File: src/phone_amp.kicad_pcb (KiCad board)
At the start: 2 copper layers, 11.6 x 56.1 mm, 41 parts, among them J1 M_USB_B, J2 PJ313D, J3 PJ313D, J4 RJ9_4P4C, J5 RJ9_4P4C, SW1 SWITCH_INV, U1 TPA6139A2, U2 MCP6024, U3 TC1017

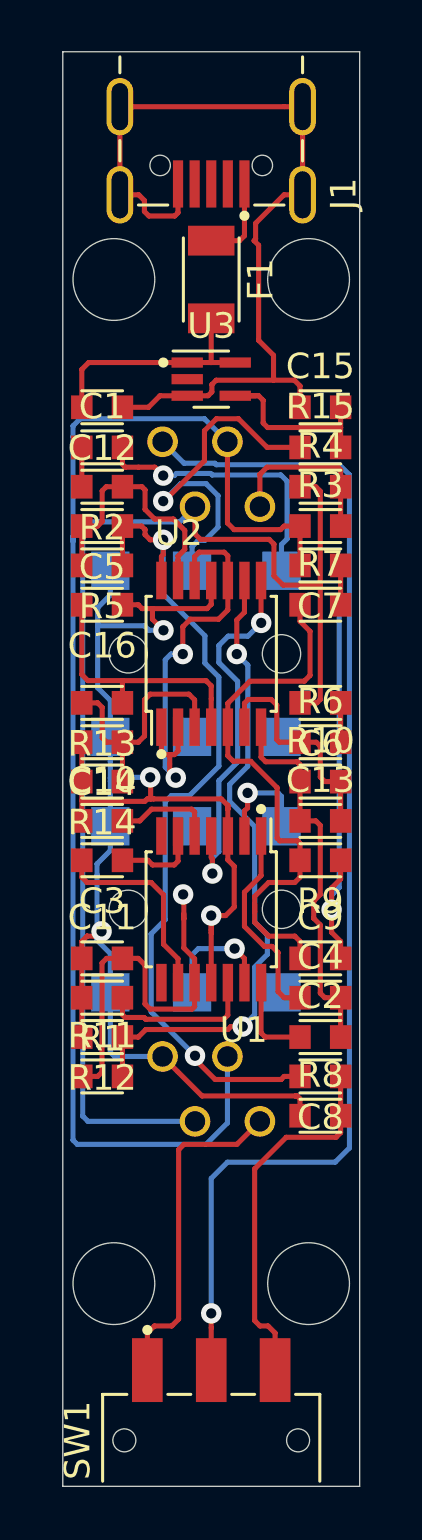
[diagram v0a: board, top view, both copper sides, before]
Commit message: Made modifications to pcb.
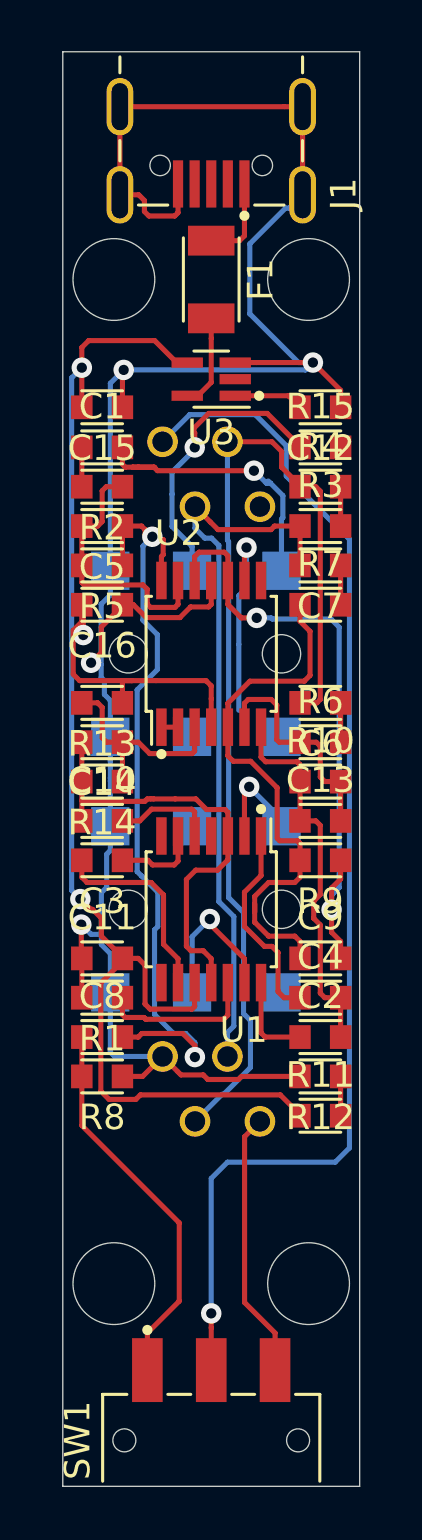
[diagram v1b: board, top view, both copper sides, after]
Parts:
- moved R11 8.68 mm to (144.0, 121.0)
- moved R8 8.68 mm to (135.4, 119.5), turned to 180 degrees
- moved C8 8.68 mm to (135.4, 118.0), turned to 0 degrees
- moved R12 8.68 mm to (144.0, 119.5)
- moved C12 8.54 mm to (144.0, 93.3)
- moved C15 8.54 mm to (135.4, 93.3), turned to 180 degrees
- turned U3 to 90 degrees
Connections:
- J1 pad 2: (no net) -> Net-(J1-Pad2)
- J1 pad 3: (no net) -> Net-(J1-Pad3)
- J1 pad 4: (no net) -> Net-(J1-Pad4)
- J2 pad 1: (no net) -> Net-(J2-Pad1)
- J2 pad 2: (no net) -> Net-(J2-Pad2)
- J3 pad 1: (no net) -> Net-(J3-Pad1)
- J3 pad 5: (no net) -> Net-(J3-Pad5)
- J5 pad 2: HS_SPK_N -> HS_SPK_P
- J5 pad 3: HS_SPK_P -> HS_SPK_N
- SW1 pad 1: HS_MIC_P -> HP_MIC_OUT
- SW1 pad 3: HP_MIC_OUT -> HS_MIC_P
- U1 pad 7: (no net) -> Net-(U1-Pad7)
- U1 pad 8: (no net) -> Net-(U1-Pad8)
- U3 pad 2: (no net) -> Net-(U3-Pad2)
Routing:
- net +3V3: track 33.4 -> 63.9 mm, vias 1 -> 3
- net HS_SPK_P: track 51.5 -> 28.5 mm
- net Net-(R11-Pad2): track 25.5 -> 9.45 mm, vias 2 -> 1
- net HP_MUTE: track 14.8 -> 0.00 mm, vias 2 -> 0
- net HS_SPK_N: track 49.7 -> 41.7 mm
- net VGND: track 32.7 -> 25.0 mm, vias 3 -> 2
- net GND: track 103.9 -> 109.7 mm
- net Net-(C12-Pad2): track 9.33 -> 6.38 mm
- net HP_MIC_BIAS: track 14.0 -> 11.3 mm
- net HS_MIC_P: track 13.2 -> 10.5 mm
- net Net-(C5-Pad1): track 33.0 -> 31.0 mm
- net Net-(C14-Pad1): track 10.1 -> 8.45 mm
- net HP_SPK_R: track 4.73 -> 6.23 mm
- net HP_MIC_OUT: track 14.5 -> 15.1 mm

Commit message: Made some pcb changes.
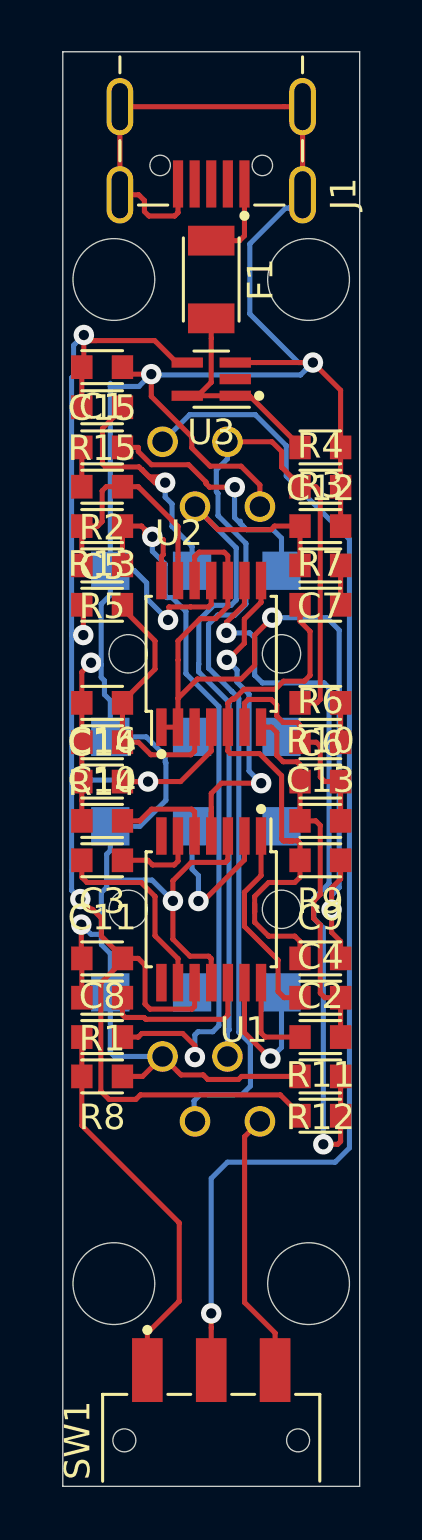
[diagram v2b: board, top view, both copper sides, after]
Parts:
- moved R15 8.68 mm to (135.4, 93.3), turned to 180 degrees
- moved C16 6.92 mm to (135.4, 108.0), turned to 0 degrees
- moved R13 3.84 mm to (135.4, 101.0), turned to 0 degrees
- moved C12 1.57 mm to (144.0, 94.9)
- moved C15 1.57 mm to (135.4, 91.7)
- moved R14 1.54 mm to (135.4, 106.4)
- moved C14 1.54 mm to (135.4, 104.9)
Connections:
- J1 pad 2: Net-(J1-Pad2) -> (no net)
- J1 pad 3: Net-(J1-Pad3) -> (no net)
- J1 pad 4: Net-(J1-Pad4) -> (no net)
- J2 pad 1: Net-(J2-Pad1) -> (no net)
- J2 pad 2: Net-(J2-Pad2) -> (no net)
- J3 pad 1: Net-(J3-Pad1) -> HP_SPK_R
- J3 pad 2: HP_SPK_R -> (no net)
- J3 pad 5: Net-(J3-Pad5) -> HP_SPK_L
- J3 pad 6: HP_SPK_L -> (no net)
- U1 pad 7: Net-(U1-Pad7) -> (no net)
- U1 pad 8: Net-(U1-Pad8) -> (no net)
- U3 pad 2: Net-(U3-Pad2) -> (no net)
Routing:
- net Net-(R11-Pad2): track 9.45 -> 29.7 mm, vias 1 -> 2
- net HP_MUTE: track 0.00 -> 13.8 mm, vias 0 -> 2
- net GND: track 109.7 -> 123.1 mm, vias 4 -> 6
- net VGND: track 25.0 -> 34.8 mm
- net HS_SPK_N: track 41.7 -> 47.1 mm
- net Net-(C12-Pad2): track 6.38 -> 8.94 mm
- net HP_SPK_L: track 4.07 -> 6.43 mm
- net Net-(C14-Pad1): track 8.45 -> 10.5 mm
- net HP_MIC: track 11.4 -> 10.0 mm
- net HP_MIC_BIAS: track 11.3 -> 9.94 mm
- net HS_SPK_P: track 28.5 -> 29.8 mm
- net Net-(C5-Pad2): track 10.6 -> 9.41 mm
- net Net-(C9-Pad1): track 21.5 -> 22.1 mm
- net +3V3: track 63.9 -> 63.5 mm, vias 3 -> 4
